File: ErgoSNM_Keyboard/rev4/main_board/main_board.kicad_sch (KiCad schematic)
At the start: 19 parts, among them J1 Conn_MouseSensor, J2 Conn_CoreBoard, J3 Conn_MouseSensor, J4 Conn_Batt, J5 Conn_Batt, J6 Conn_CoreBoard, SW1 SW_DPDT_x2, SW2 RESET, SW3 RESET, SW4 SW_DPDT_x2

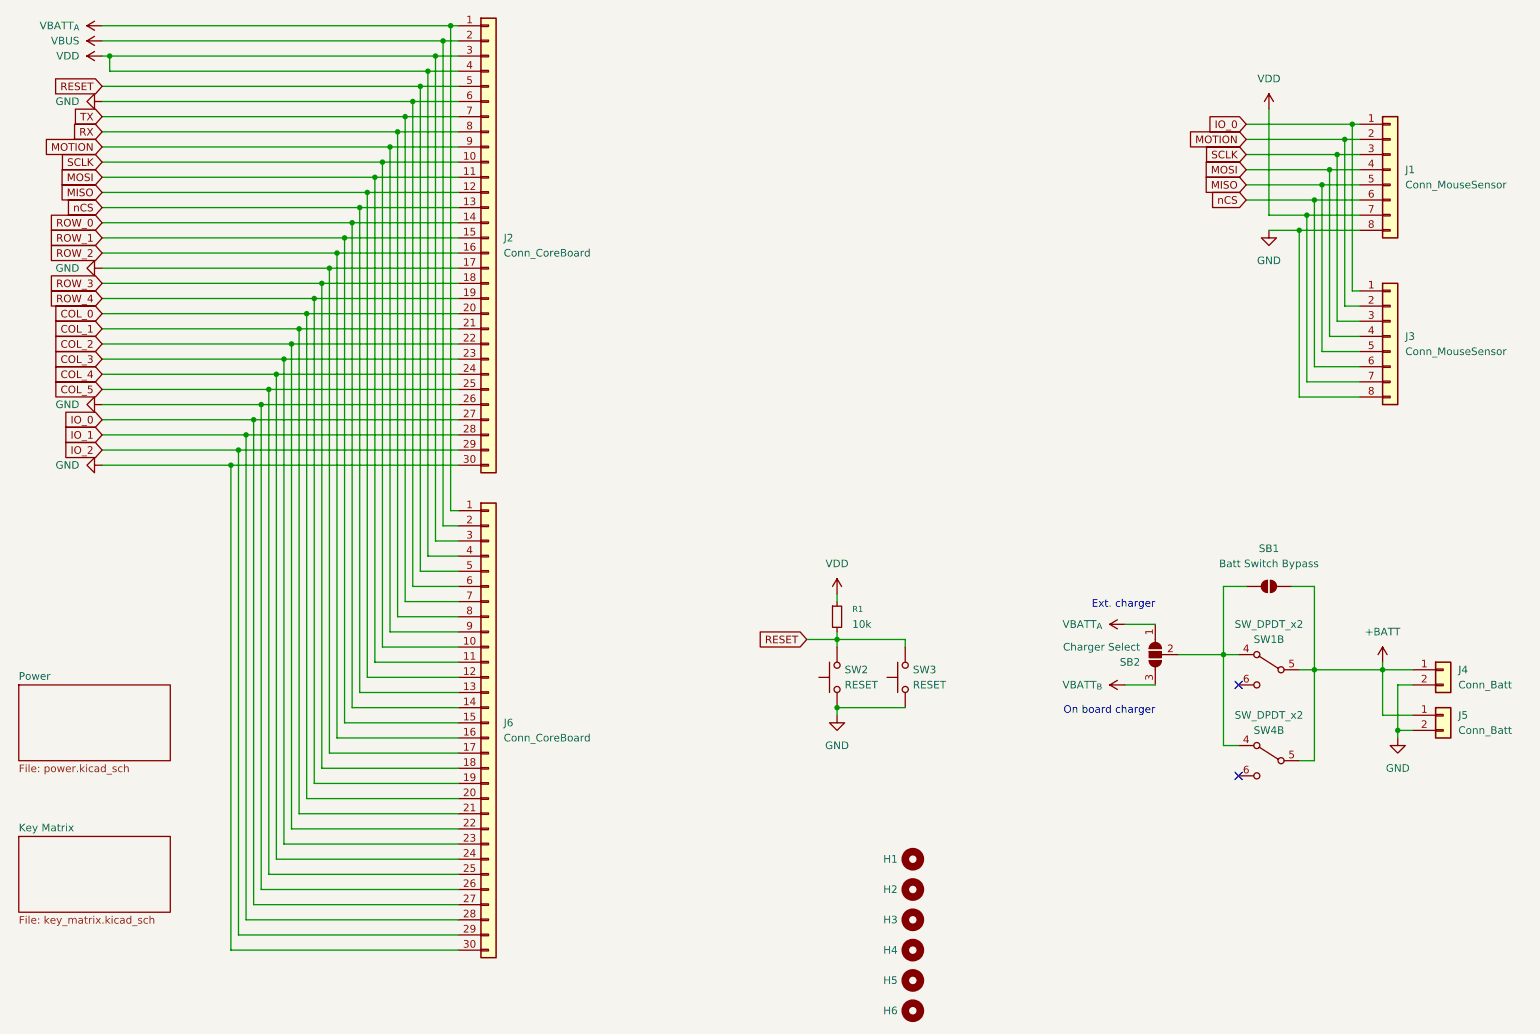
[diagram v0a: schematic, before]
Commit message: feat: update main board layout
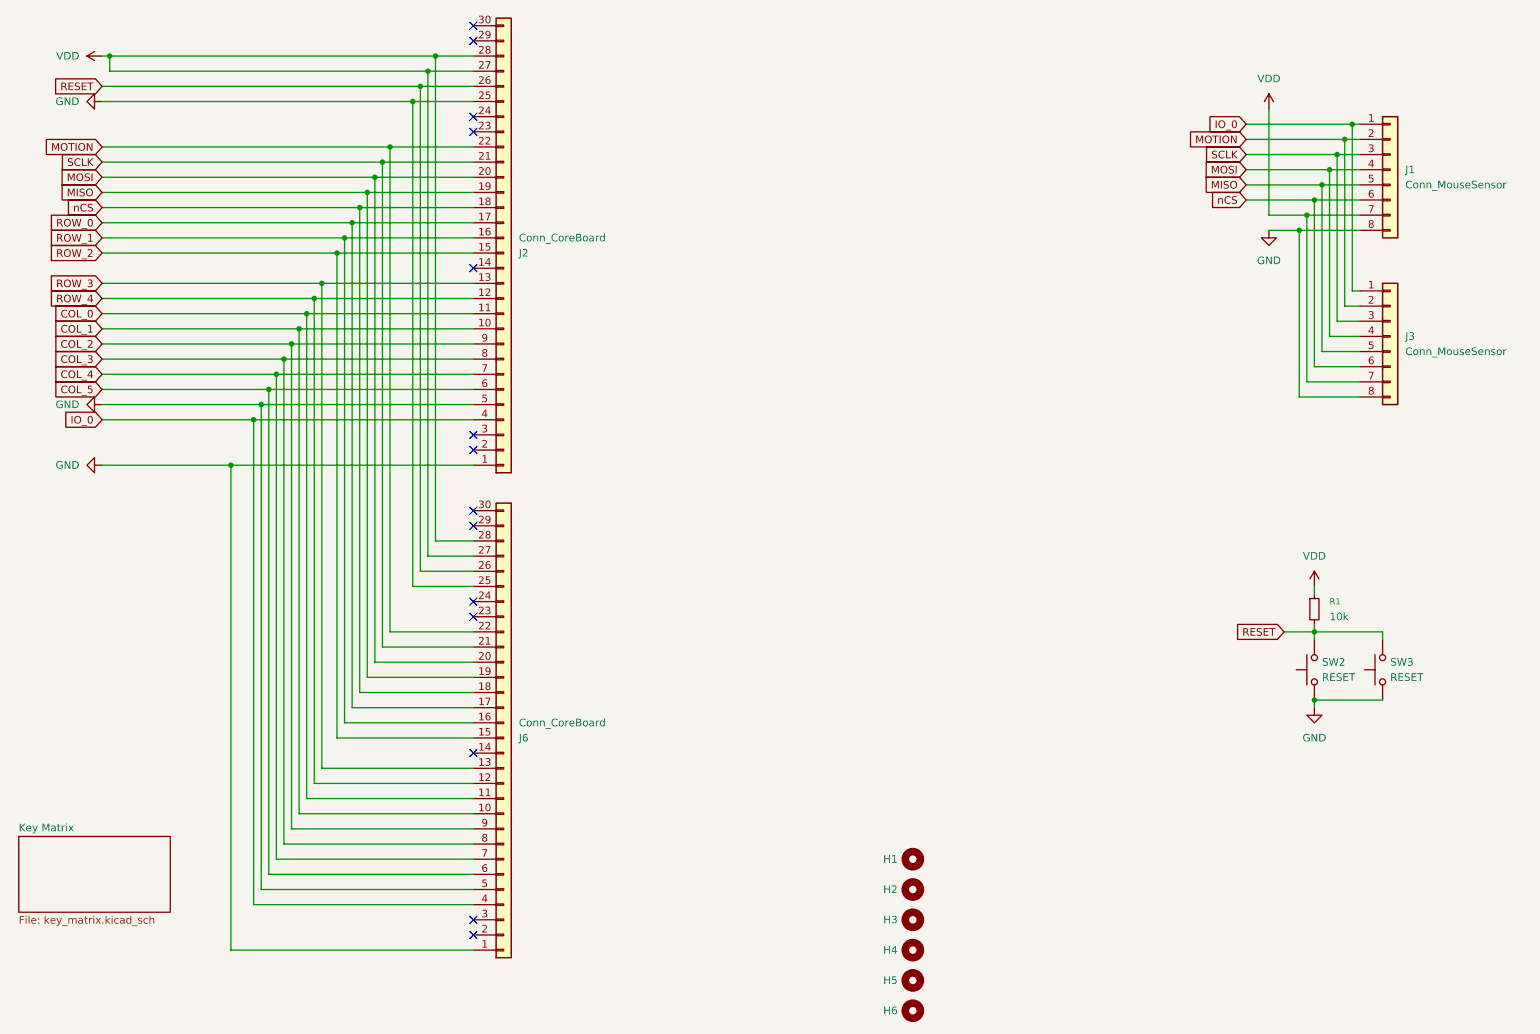
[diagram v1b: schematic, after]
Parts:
- removed J4, J5: Conn_Batt, Connector_JST:JST_PH_S2B-PH-SM4-TB_1x02-1MP_P2.00mm_Horizontal, symbol Connector_Generic:Conn_01x02
- removed SB1: Batt Switch Bypass, Jumper:SolderJumper-2_P1.3mm_Open_TrianglePad1.0x1.5mm, symbol Jumper:SolderJumper_2_Open
- removed SB2: Charger Select, Jumper:SolderJumper-3_P2.0mm_Open_TrianglePad1.0x1.5mm_NumberLabels, symbol Jumper:SolderJumper_3_Open
- removed SW1, SW4: SW_DPDT_x2, ErgoSNM_Keyboard:MSKT-22D14-T, symbol Switch:SW_DPDT_x2
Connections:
- net IO_1 is gone; now on net VDD: J2.28 (Pin_28), J6.28 (Pin_28)
- net RX is gone; now on net COL_3: J2.8 (Pin_8), J6.8 (Pin_8)
- net TX is gone; now on net COL_4: J2.7 (Pin_7), J6.7 (Pin_7)
- net VBATT_{A} is gone; now on net GND: J2.1 (Pin_1), J6.1 (Pin_1)
- net COL_0: now also J2.11 (Pin_11), J6.11 (Pin_11); no longer J2.20 (Pin_20), J6.20 (Pin_20)
- net COL_1: now also J2.10 (Pin_10), J6.10 (Pin_10); no longer J2.21 (Pin_21), J6.21 (Pin_21)
- net COL_2: now also J2.9 (Pin_9), J6.9 (Pin_9); no longer J2.22 (Pin_22), J6.22 (Pin_22)
- net COL_3: no longer J2.23 (Pin_23), J6.23 (Pin_23)
- net COL_4: no longer J2.24 (Pin_24), J6.24 (Pin_24)
- net COL_5: now also J2.6 (Pin_6), J6.6 (Pin_6); no longer J2.25 (Pin_25), J6.25 (Pin_25)
- net GND: now also J2.25 (Pin_25), J2.5 (Pin_5), J6.25 (Pin_25), J6.5 (Pin_5); no longer J2.17 (Pin_17), J2.26 (Pin_26), J2.30 (Pin_30), J2.6 (Pin_6), J6.17 (Pin_17), J6.26 (Pin_26), J6.30 (Pin_30), J6.6 (Pin_6)
- net IO_0: now also J2.4 (Pin_4), J6.4 (Pin_4); no longer J2.27 (Pin_27), J6.27 (Pin_27)
- net MISO: now also J2.19 (Pin_19), J6.19 (Pin_19); no longer J2.12 (Pin_12), J6.12 (Pin_12)
- net MOSI: now also J2.20 (Pin_20), J6.20 (Pin_20); no longer J2.11 (Pin_11), J6.11 (Pin_11)
- net MOTION: now also J2.22 (Pin_22), J6.22 (Pin_22); no longer J2.9 (Pin_9), J6.9 (Pin_9)
- net RESET: now also J2.26 (Pin_26), J6.26 (Pin_26); no longer J2.5 (Pin_5), J6.5 (Pin_5)
- net ROW_0: now also J2.17 (Pin_17), J6.17 (Pin_17); no longer J2.14 (Pin_14), J6.14 (Pin_14)
- net ROW_1: now also J2.16 (Pin_16), J6.16 (Pin_16); no longer J2.15 (Pin_15), J6.15 (Pin_15)
- net ROW_2: now also J2.15 (Pin_15), J6.15 (Pin_15); no longer J2.16 (Pin_16), J6.16 (Pin_16)
- net ROW_3: now also J2.13 (Pin_13), J6.13 (Pin_13); no longer J2.18 (Pin_18), J6.18 (Pin_18)
- net ROW_4: now also J2.12 (Pin_12), J6.12 (Pin_12); no longer J2.19 (Pin_19), J6.19 (Pin_19)
- net SCLK: now also J2.21 (Pin_21), J6.21 (Pin_21); no longer J2.10 (Pin_10), J6.10 (Pin_10)
- net VDD: now also J2.27 (Pin_27), J6.27 (Pin_27); no longer J2.3 (Pin_3), J2.4 (Pin_4), J6.3 (Pin_3), J6.4 (Pin_4)
- net nCS: now also J2.18 (Pin_18), J6.18 (Pin_18); no longer J2.13 (Pin_13), J6.13 (Pin_13)
- net IO_2: no longer names the net of J2.29 (Pin_29)
- net IO_2: no longer J6.29 (Pin_29)
- net VBUS: no longer names the net of J2.2 (Pin_2)
- net VBUS: no longer J6.2 (Pin_2)
- no-connect marks 2 -> 14
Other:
- removed sheet Power
- note removed: "Ext. charger"
- note removed: "On board charger"
- moved on the sheet: J2, J6, R1, SW2, SW3
